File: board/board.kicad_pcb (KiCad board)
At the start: 2 copper layers, 21 x 13 mm, 1 part

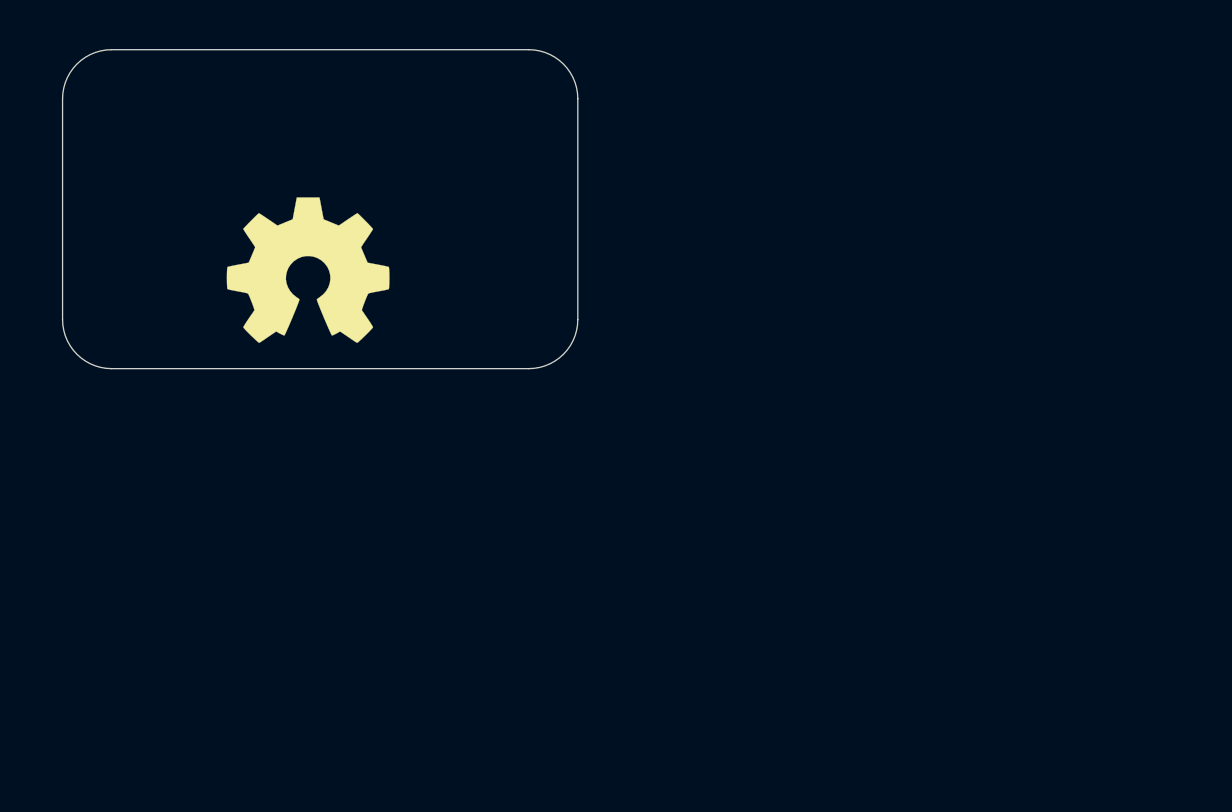
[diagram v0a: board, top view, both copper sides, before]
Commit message: initial
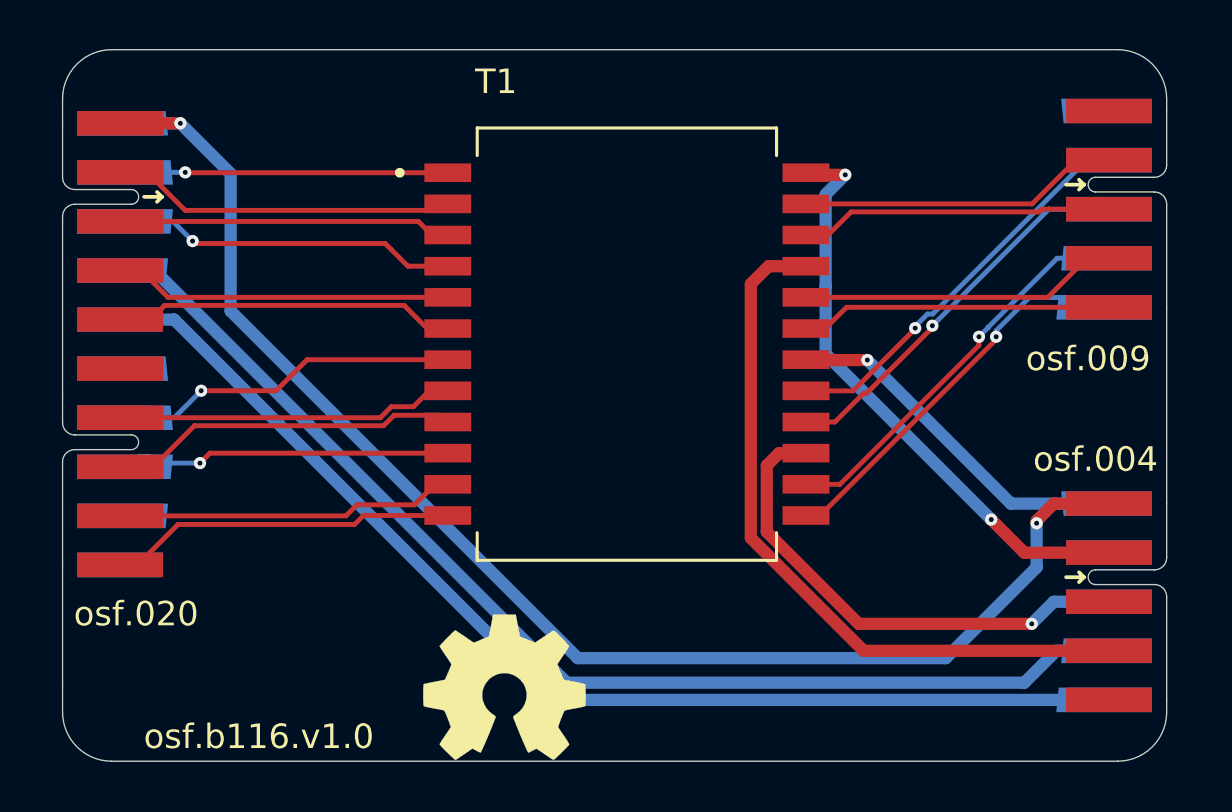
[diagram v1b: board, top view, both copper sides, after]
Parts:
- added J1: 020_1000BASE-T_with_CT, on_edge:on_edge_2x10_device, F.Cu at (140.0, 97.0)
- added J2: 009_1000BASE-T, on_edge:on_edge_2x05_host, F.Cu at (185.0, 96.5)
- added J3: 004_BASE-T_CT, on_edge:on_edge_2x05_host, F.Cu at (185.0, 112.5)
- added T1: PT61020EL, b116:XFMR_PT61020EL, F.Cu at (163.0, 102.0)
- moved LOGO1 18.8 mm to (158.0, 116.0)
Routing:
- net GND: track 0.00 -> 58.7 mm, vias 0 -> 2
- net /3.3V: track 0.00 -> 47.7 mm
- net /5V: track 0.00 -> 46.6 mm
- net /eth_magnetics/CT2: track 0.00 -> 29.4 mm
- net /eth_magnetics/CT1: track 0.00 -> 24.2 mm, vias 0 -> 2
- net /eth_magnetics/CT4: track 0.00 -> 20.4 mm, vias 0 -> 1
- net /eth_magnetics/RXD2+: track 0.00 -> 16.3 mm, vias 0 -> 1
- net /eth_magnetics/TXD2+: track 0.00 -> 16.3 mm, vias 0 -> 1
- net /eth_magnetics/RXD2-: track 0.00 -> 16.3 mm, vias 0 -> 1
- net /eth_magnetics/TXD2-: track 0.00 -> 16.0 mm, vias 0 -> 1
- net /eth_magnetics/CT3: track 0.00 -> 14.7 mm, vias 0 -> 1
- net /eth_magnetics/TCT2: track 0.00 -> 14.6 mm, vias 0 -> 1
- net /eth_magnetics/RCT1: track 0.00 -> 14.4 mm, vias 0 -> 1
- net /eth_magnetics/TX2-: track 0.00 -> 14.3 mm
- net /eth_magnetics/RX2-: track 0.00 -> 14.2 mm
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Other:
- board size 21 x 13 mm -> 45 x 29 mm
- board text added: "osf.004"
- board text added: "osf.009"
- board text added: "osf.020"
- board text added: "osf.b116.v1.0"
